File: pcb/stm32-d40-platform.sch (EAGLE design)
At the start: 84 parts, among them IC1 STM32F103C8, IC2 TODO AMIS30663CANG2G, IC3 STM32F103C8, J1 DIP-40, Q1 8MHz, Q2 8MHz, SW1 KSS-2EG4430, SW2 KSS-2EG4430, X1 DG3XX-03-3.5

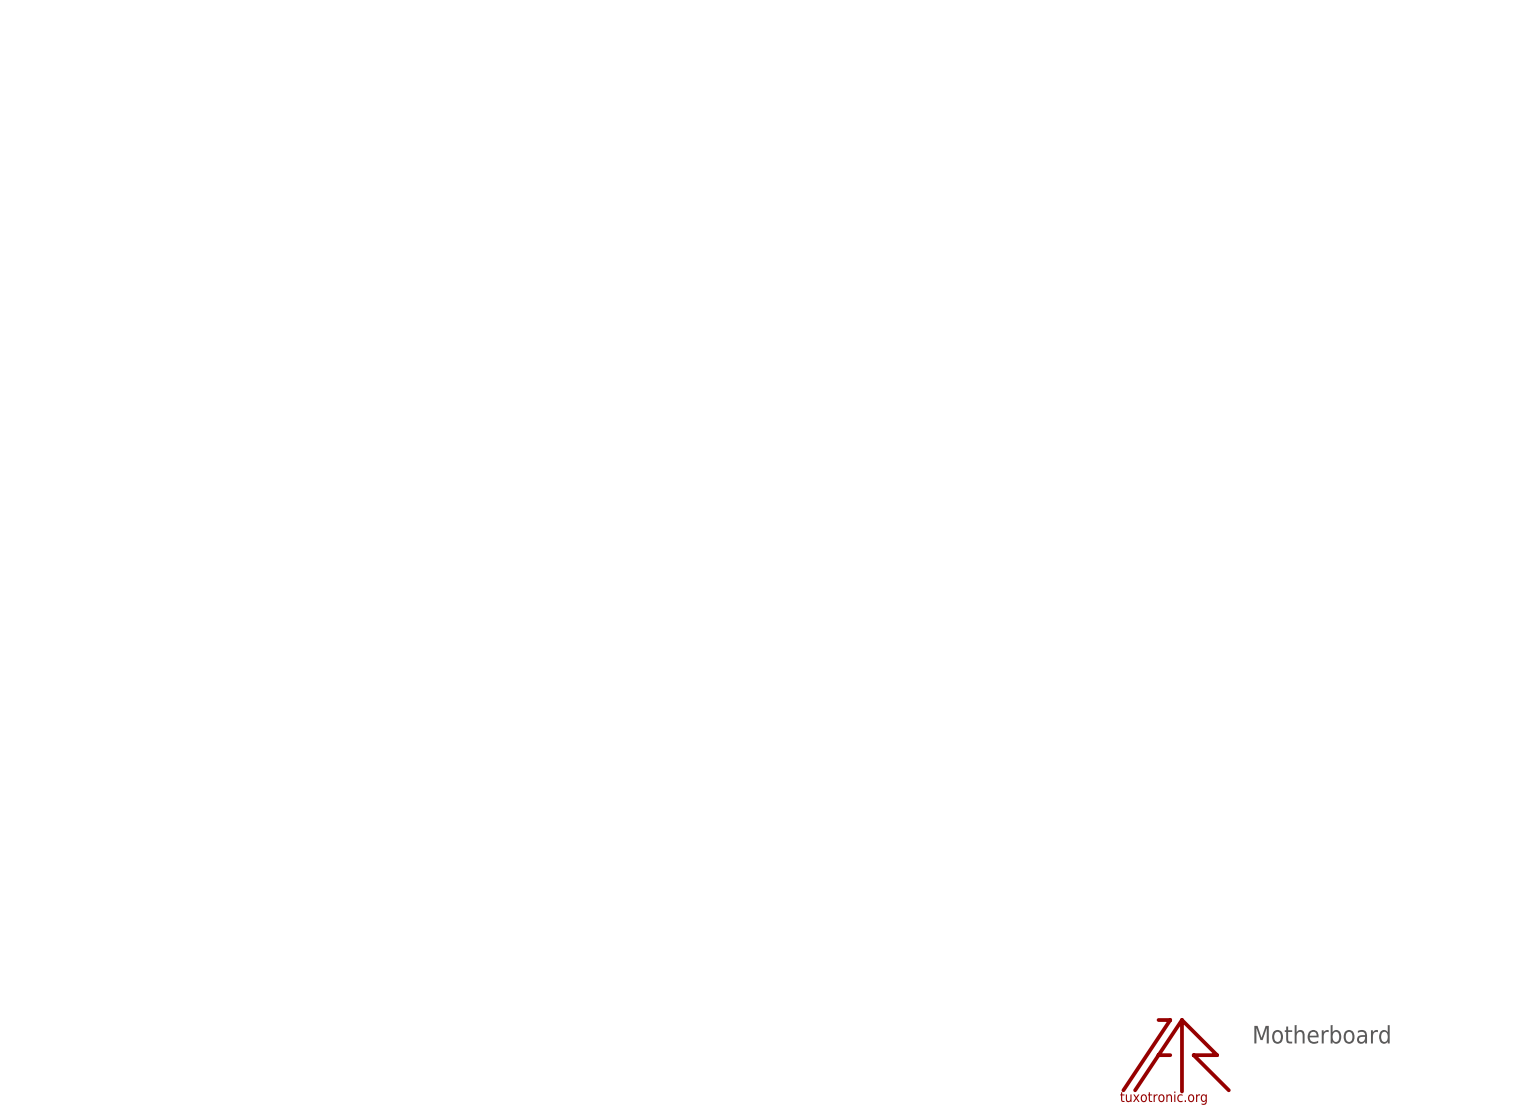
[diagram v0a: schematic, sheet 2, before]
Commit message: motherboard in progress
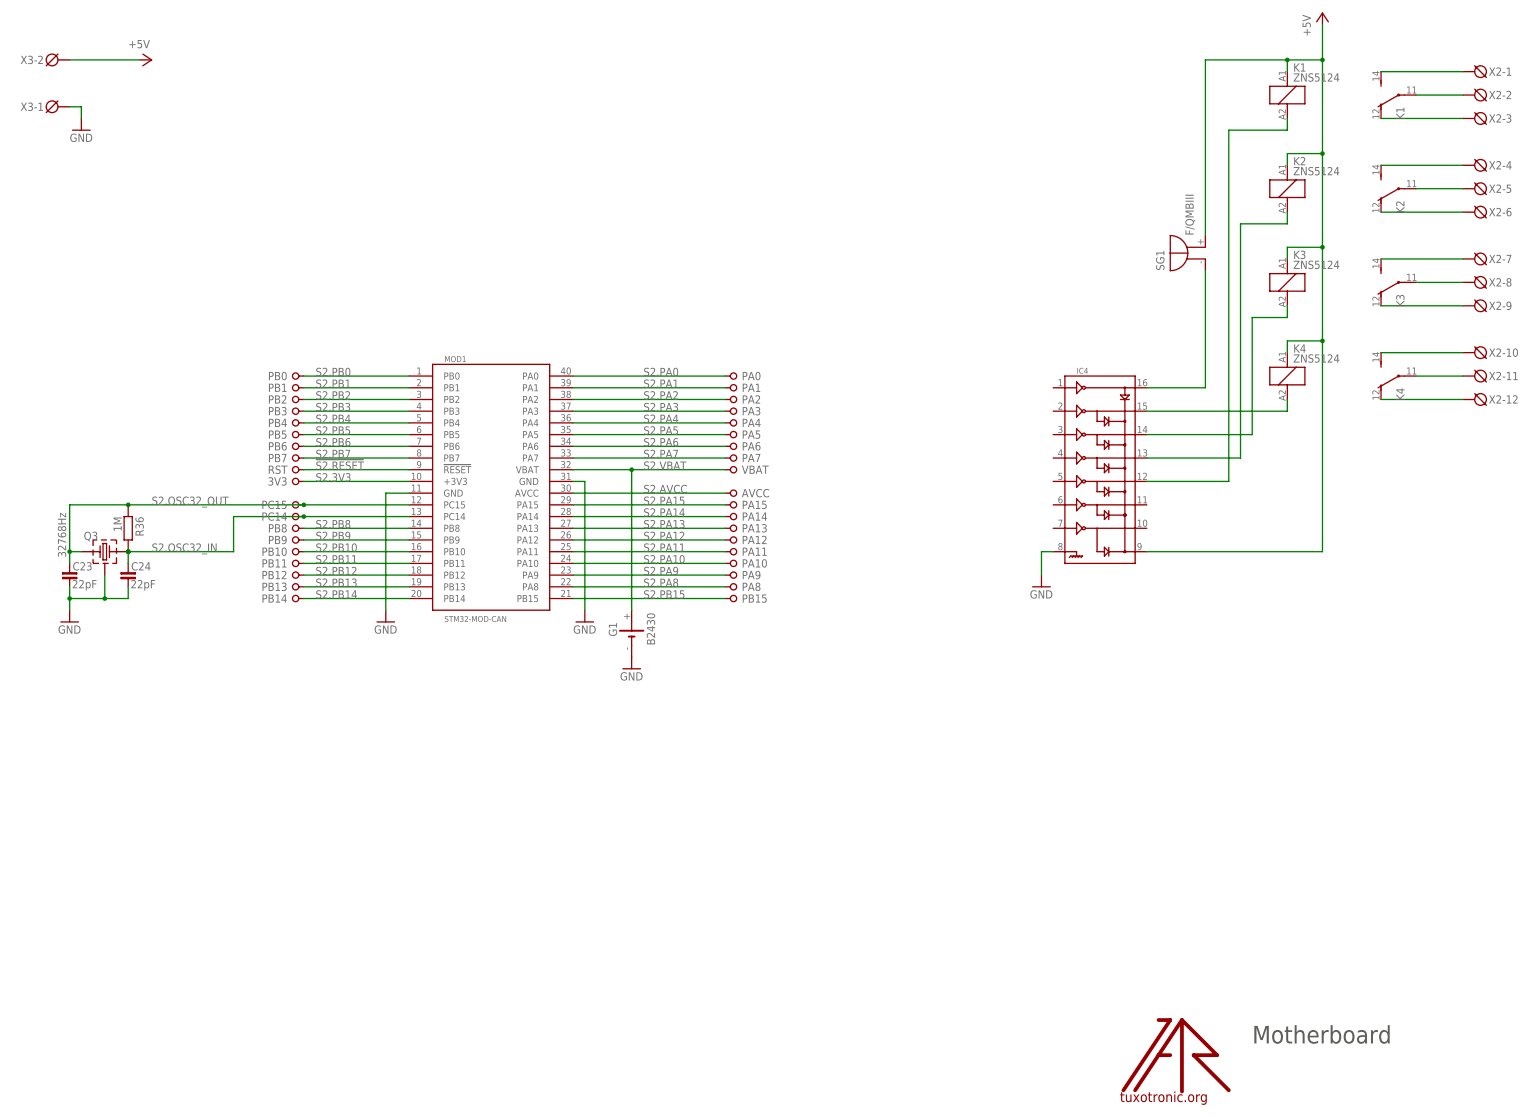
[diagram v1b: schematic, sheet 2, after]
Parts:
- added 3V3, AVCC, PA0, PA1, PA10, PA11, PA12, PA13, PA14, PA15, PA2, PA3, PA4, PA5, PA6, PA7, PA8, PA9, PB0, PB1, PB10, PB11, PB12, PB13, PB14, PB15, PB2, PB3, PB4, PB5, PB6, PB7, PB8, PB9, PC14, PC15, RST, VBAT: (no value), pinhead-fixdrills:PIN-1X1_2.54
- added C23, C24: 22pF, rc-master-smd:C_0603
- added G1: B2430, battery:B2430
- added IC4: (no value), transistor-arrays:ULN2003D
- added K1, K2, K3, K4: ZNS5124, myrelays:ZNS5124
- added MOD1: STM32-MOD-CAN, stamp:STM32-MOD-CAN
- added Q3: 32768Hz, crystal:CRSTL3-
- added R36: 1M, rc-master-smd:R_0603
- added SG1: F/QMBIII, buzzer:F/QMBIII
- added X2: DG3XX-12-5.0, degson:DG3XX-12-5.0
- added X3: DG3XX-02-5.0, degson:DG3XX-02-5.0
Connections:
- new net !S2.RESET: MOD1.!RESET, RST.1
- new net N$366: IC4.15, K41.2
- new net N$367: IC4.14, K31.2
- new net N$368: IC4.13, K21.2
- new net N$369: IC4.12, K11.2
- new net N$370: IC4.16, SG1.+
- new net N$64: K12.S, X2-1.KL
- new net N$65: K12.P, X2-2.KL
- new net N$66: K12.O, X2-3.KL
- new net N$67: K22.S, X2-4.KL
- new net N$68: K22.P, X2-5.KL
- new net N$69: K22.O, X2-6.KL
- new net N$70: K32.S, X2-7.KL
- new net N$71: K32.P, X2-8.KL
- new net N$72: K32.O, X2-9.KL
- new net N$73: K42.S, X2-10.KL
- new net N$74: K42.P, X2-11.KL
- new net N$75: K42.O, X2-12.KL
- new net S2.3V3: 3V3.1, MOD1.+3V3
- new net S2.AVCC: AVCC.1, MOD1.AVCC
- new net S2.OSC32_IN: C24.1, MOD1.PC14, PC14.1, Q3.2, R36.2
- new net S2.OSC32_OUT: C23.1, MOD1.PC15, PC15.1, Q3.1, R36.1
- new net S2.PA0: MOD1.PA0, PA0.1
- new net S2.PA1: MOD1.PA1, PA1.1
- new net S2.PA10: MOD1.PA10, PA10.1
- new net S2.PA11: MOD1.PA11, PA11.1
- new net S2.PA12: MOD1.PA12, PA12.1
- new net S2.PA13: MOD1.PA13, PA13.1
- new net S2.PA14: MOD1.PA14, PA14.1
- new net S2.PA15: MOD1.PA15, PA15.1
- new net S2.PA2: MOD1.PA2, PA2.1
- new net S2.PA3: MOD1.PA3, PA3.1
- new net S2.PA4: MOD1.PA4, PA4.1
- new net S2.PA5: MOD1.PA5, PA5.1
- new net S2.PA6: MOD1.PA6, PA6.1
- new net S2.PA7: MOD1.PA7, PA7.1
- new net S2.PA8: MOD1.PA8, PA8.1
- new net S2.PA9: MOD1.PA9, PA9.1
- new net S2.PB0: MOD1.PB0, PB0.1
- new net S2.PB1: MOD1.PB1, PB1.1
- new net S2.PB10: MOD1.PB10, PB10.1
- new net S2.PB11: MOD1.PB11, PB11.1
- new net S2.PB12: MOD1.PB12, PB12.1
- new net S2.PB13: MOD1.PB13, PB13.1
- new net S2.PB14: MOD1.PB14, PB14.1
- new net S2.PB15: MOD1.PB15, PB15.1
- new net S2.PB2: MOD1.PB2, PB2.1
- new net S2.PB3: MOD1.PB3, PB3.1
- new net S2.PB4: MOD1.PB4, PB4.1
- new net S2.PB5: MOD1.PB5, PB5.1
- new net S2.PB6: MOD1.PB6, PB6.1
- new net S2.PB7: MOD1.PB7, PB7.1
- new net S2.PB8: MOD1.PB8, PB8.1
- new net S2.PB9: MOD1.PB9, PB9.1
- new net S2.VBAT: G1.+, MOD1.VBAT, VBAT.1
- net +5V: now also IC4.9, K11.1, K21.1, K31.1, K41.1, SG1.-, X3-2.KL
- net GND: now also C23.2, C24.2, G1.-, IC4.8, MOD1.GND@11, MOD1.GND@31, Q3.P$1, X3-1.KL
